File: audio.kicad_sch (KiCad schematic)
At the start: 32 parts, among them IC10 LM386

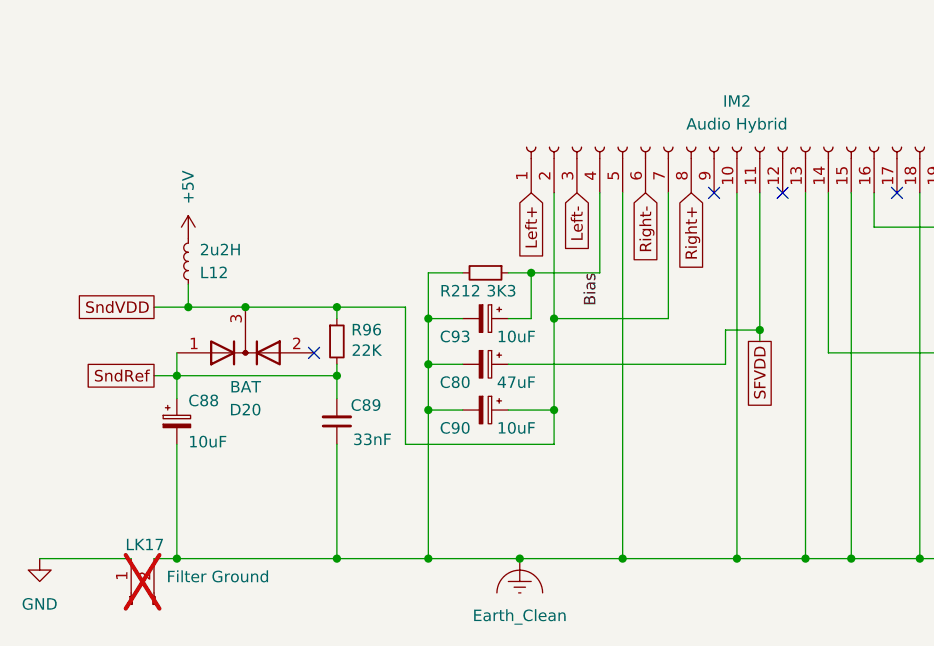
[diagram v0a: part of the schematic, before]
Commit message: yet more traces
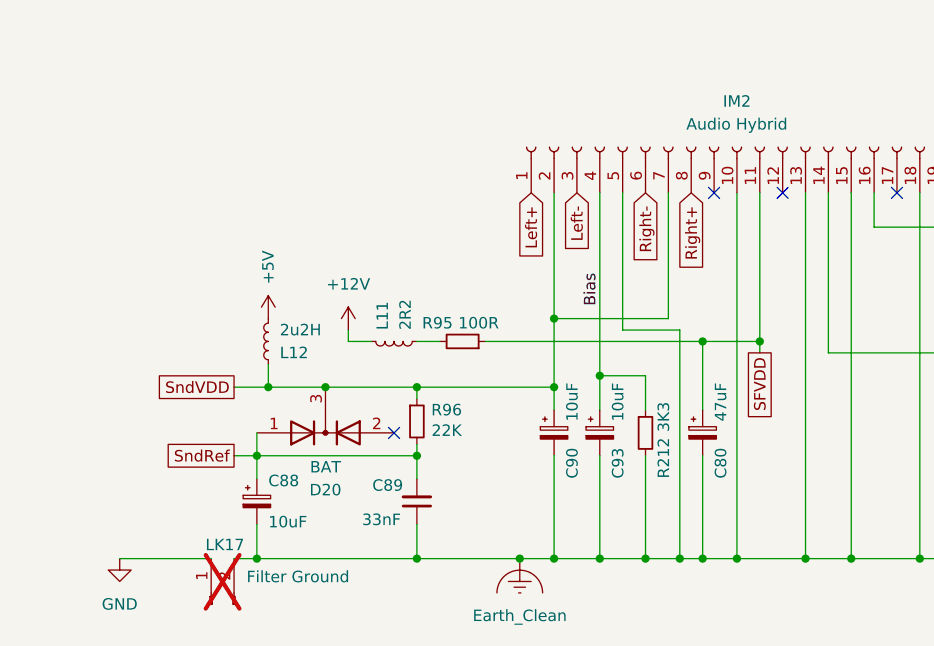
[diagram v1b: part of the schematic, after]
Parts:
- added L11: 2R2, Acorn:L_Acorn_8x3mm, symbol Device:L_Small
- added R95: 100R, Resistor_SMD:R_0805_2012Metric, symbol Device:R_Small
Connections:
- net SFVDD: now also R95.1
- new net: L11.2, R95.2
- new net +12V: L11.1
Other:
- moved on the sheet: C80, C88, C89, C90, C93, D20, L12, LK17, R212, R96
